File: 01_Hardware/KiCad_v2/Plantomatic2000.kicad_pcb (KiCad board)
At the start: 4 copper layers, 137.2 x 78 mm, 284 parts, among them J100 TYPE-C-31-M-12, J300 JST_B2B, J600 JST_B2B, J601 JST_B2B, J700 JST_B4B, J701 JST_B4B, J800 Conn_02x03_Odd_Even, J801 JST_B2B, J802 JST_B2B, J803 JST_B2B, J804 Conn_02x05_Odd_Even, J805 JST_B2B, J806 JST_B2B, J807 JST_B2B, J808 JST_B2B, Q100 UMH3N, Q200 SI7615DN-T1-GE3, Q201 SI7615DN-T1-GE3, Q202 DMP6050SSD, Q203 NVTA7002NT1G, Q300 BSS314PE, Q301 NVTA7002NT1G, Q400 SI7615DN-T1-GE3, Q401 SI7615DN-T1-GE3, Q402 NVTA7002NT1G, Q500 NVTA7002NT1G, Q600 STN3NF06L, Q601 STN3NF06L, Q700 BSS314PE, Q701 BSS314PE, Q702 NVTA7002NT1G, Q703 NVTA7002NT1G, SW800 SW_Push, SW801 SW_Push, U100 USBLC6-2P6, U101 CP2102N-A02-GQFN24, U200 CYPD3177-24LQ, U300 BQ25892, U400 BDJ2FC0WFP, U401 TLV61048, U402 NCP1117-12_SOT223, U403 XC6220B331MR, U404 XC6220B331MR, U500 DS3231M, U501 ESP32-WROOM-32E, U502 AT24CS01-SSHM

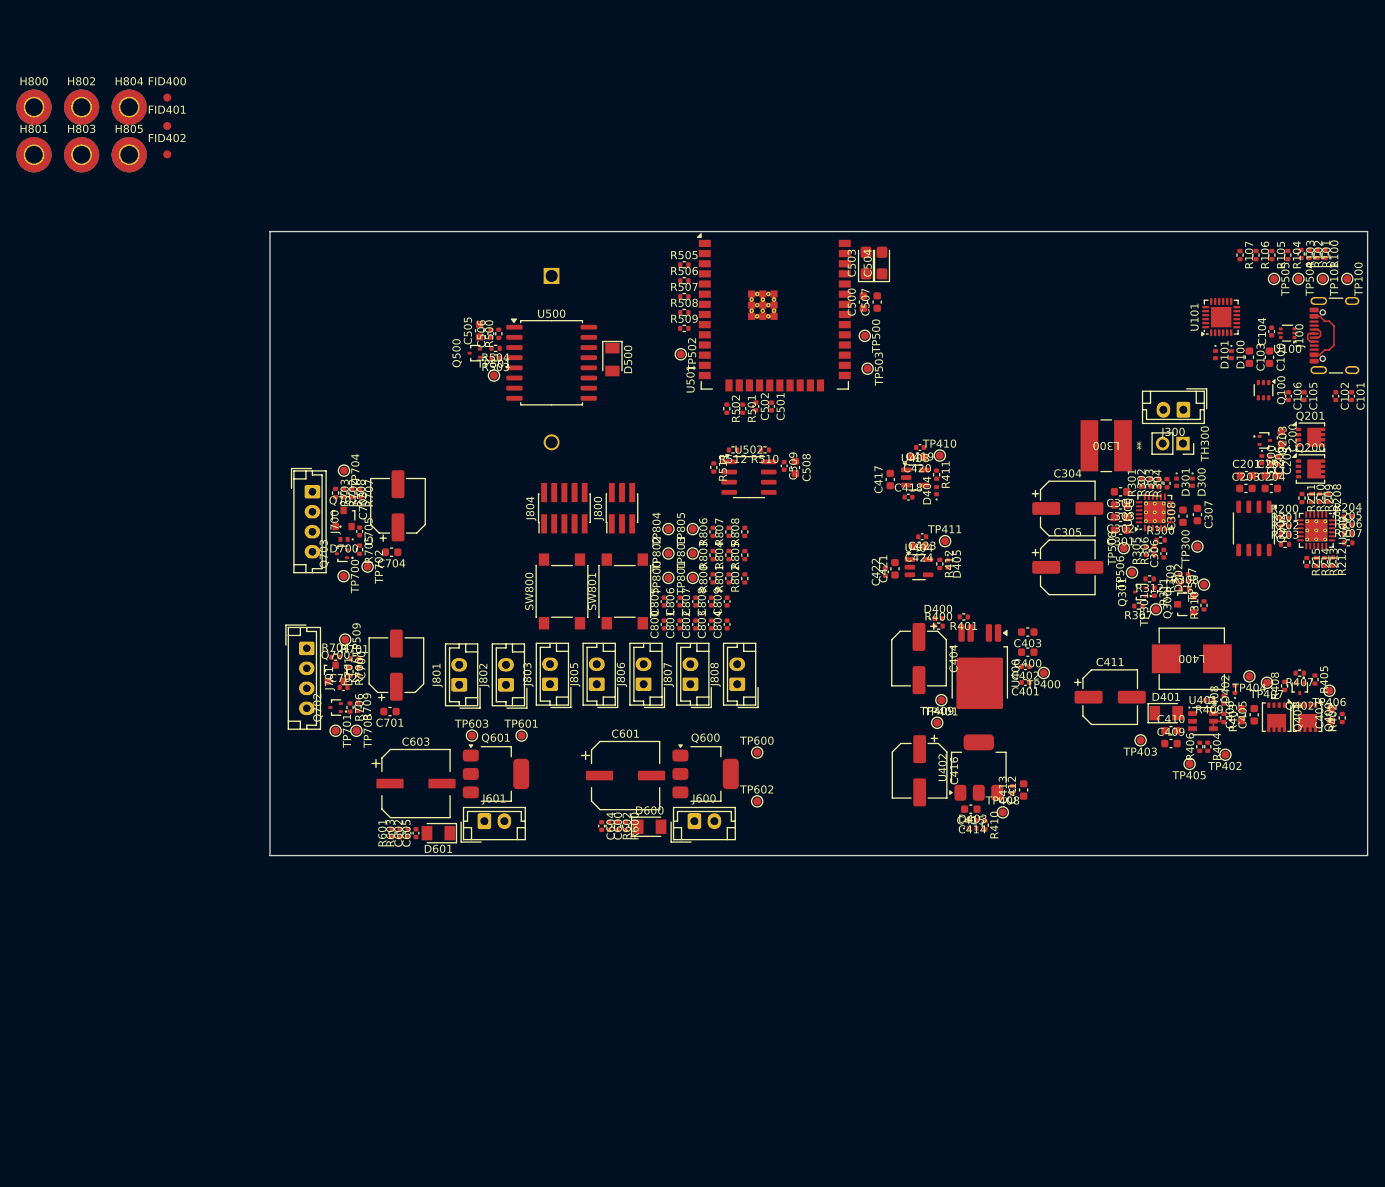
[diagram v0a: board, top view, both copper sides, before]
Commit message: USB-C and Serial PCB routing done
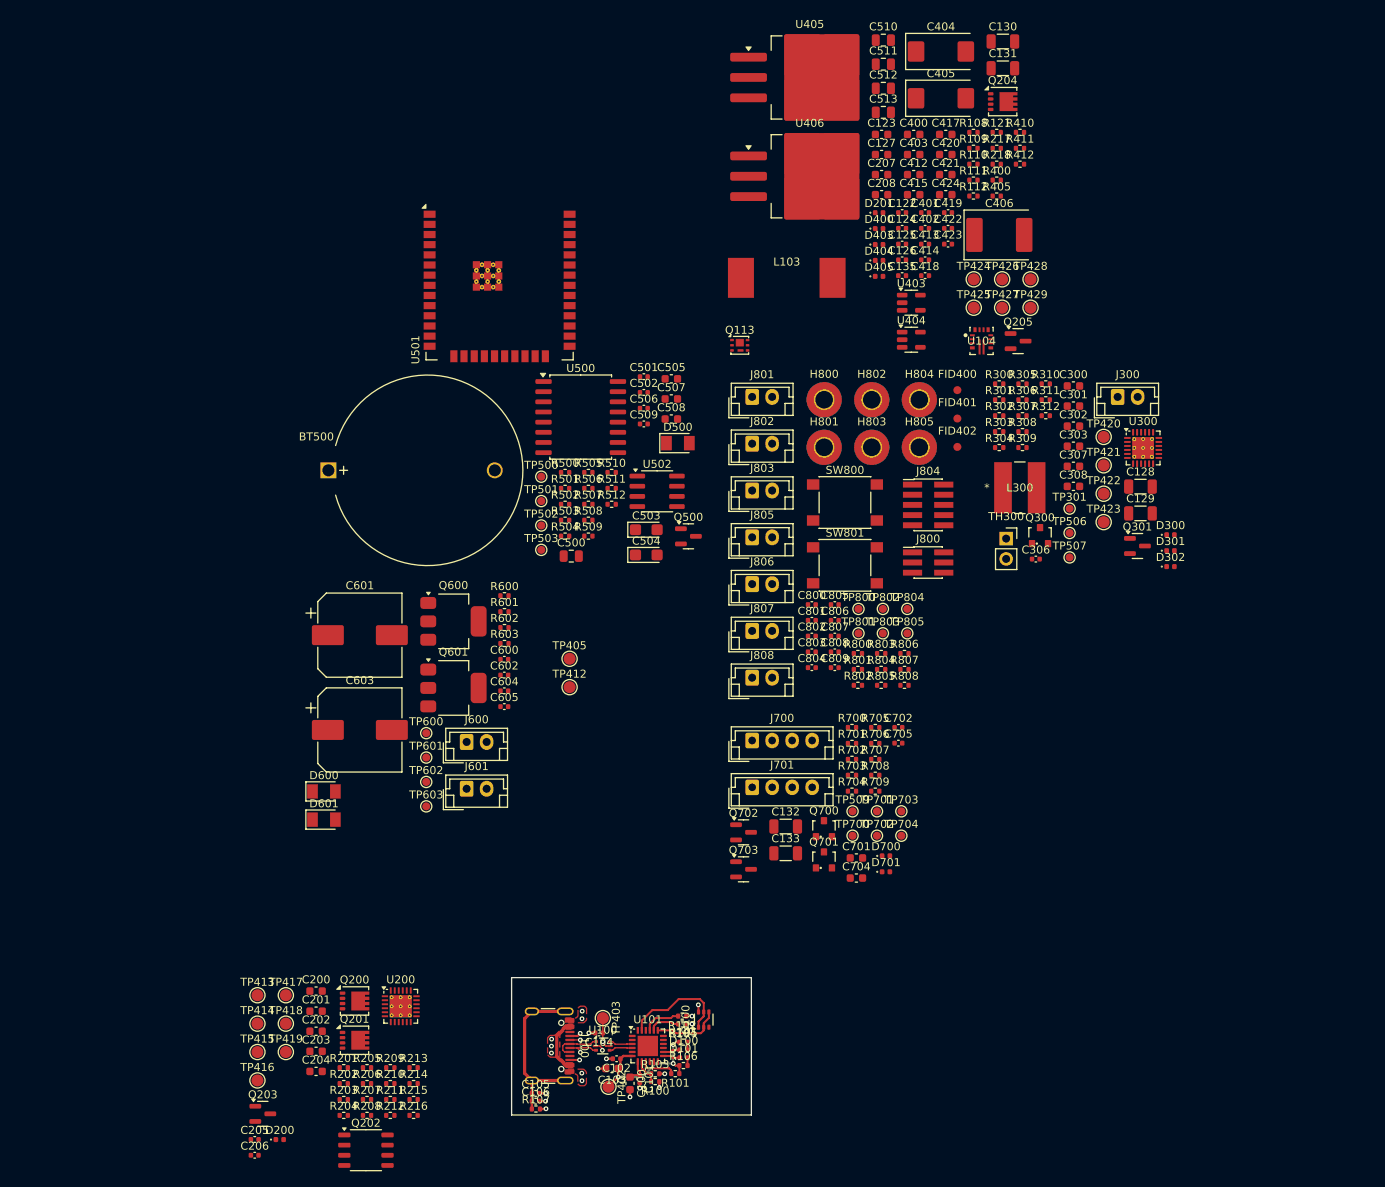
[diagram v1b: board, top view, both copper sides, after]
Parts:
- removed C304, C305, C411, C416, C700, C703: 47uF, Capacitor_SMD:CP_Elec_6.3x5.8
- removed C407, C409: 1uF, Capacitor_SMD:C_0603_1608Metric
- removed C408: 100nF, Capacitor_SMD:C_0402_1005Metric
- removed C410: 10uF, Capacitor_SMD:C_0603_1608Metric
- removed D401: SBR3U40S1F, Custom_Global_Footprints:SBR3U40S1F-7
- removed D402: NCD0402G1, Custom_Global_Footprints:SML-P13PTT_LED_0402_1005Metric
- removed L400: ETQ-P5M100YFM, Custom_Global_Footprints:ETQ-P5M100YFM
- removed Q400, Q401: SI7615DN-T1-GE3, Package_SON:Diodes_PowerDI3333-8
- removed Q402: NVTA7002NT1G, Custom_Global_Footprints:NVTA7002N
- removed R200, R401, R402, R403, R407: 10K, Resistor_SMD:R_0402_1005Metric
- removed R404: 1M, Resistor_SMD:R_0402_1005Metric
- removed R406: 64K9, Resistor_SMD:R_0402_1005Metric
- removed R408: 22K1, Resistor_SMD:R_0402_1005Metric
- removed R409: 1K, Resistor_SMD:R_0402_1005Metric
- removed TP100, TP101, TP404, TP406, TP407, TP410, TP411, TP504, TP505, TP508: ~, TestPoint:TestPoint_Pad_D1.0mm
- removed TP300: +VBAT, TestPoint:TestPoint_Pad_D1.0mm
- removed TP400, TP401, TP408, TP409: TestPoint_Small, TestPoint:TestPoint_Pad_D1.0mm
- removed U400: BDJ2FC0WFP, Package_TO_SOT_SMD:TO-252-4
- removed U401: TLV61048, Custom_Global_Footprints:TLV61048
- removed U402: NCP1117-12_SOT223, Package_TO_SOT_SMD:SOT-223
- added C122: 100nF, Capacitor_SMD:C_0402_1005Metric, F.Cu at (193.6, 46.5)
- added C123: 10uF, Capacitor_SMD:C_0603_1608Metric, F.Cu at (191.1, 36.8)
- added C124: 100nF, Capacitor_SMD:C_0402_1005Metric, F.Cu at (193.6, 48.5)
- added C125: 100pF, Capacitor_SMD:C_0402_1005Metric, F.Cu at (193.6, 50.5)
- added C126: 22nF, Capacitor_SMD:C_0402_1005Metric, F.Cu at (193.6, 52.4)
- added C127: 4.7uF, Capacitor_SMD:C_0603_1608Metric, F.Cu at (191.1, 39.3)
- added C128: 47uF, Capacitor_SMD:C_1206_3216Metric, F.Cu at (223.4, 80.8)
- added C129: 47uF, Capacitor_SMD:C_1206_3216Metric, F.Cu at (223.4, 84.1)
- added C130: 47uF, Capacitor_SMD:C_1206_3216Metric, F.Cu at (206.2, 25.1)
- added C131: 47uF, Capacitor_SMD:C_1206_3216Metric, F.Cu at (206.2, 28.5)
- added C132: 47uF, Capacitor_SMD:C_1206_3216Metric, F.Cu at (179.1, 123.3)
- added C133: 47uF, Capacitor_SMD:C_1206_3216Metric, F.Cu at (179.1, 126.6)
- added C135: 22nF, Capacitor_SMD:C_0402_1005Metric, F.Cu at (193.6, 54.4)
- added C207: 1uF, Capacitor_SMD:C_0603_1608Metric, F.Cu at (191.1, 41.8)
- added C208: 1uF, Capacitor_SMD:C_0603_1608Metric, F.Cu at (191.1, 44.3)
- added C510: 22uF, Capacitor_SMD:C_0805_2012Metric, F.Cu at (191.3, 25.0)
- added C511: 22uF, Capacitor_SMD:C_0805_2012Metric, F.Cu at (191.3, 28.0)
- added C512: 22uF, Capacitor_SMD:C_0805_2012Metric, F.Cu at (191.3, 31.0)
- added C513: 22uF, Capacitor_SMD:C_0805_2012Metric, F.Cu at (191.3, 34.0)
- added D201: NCD0402R1, LED_SMD:LED_0402_1005Metric, F.Cu at (190.7, 46.5)
- added L103: 4.7uH (SPM12565VT-4R7M-D), Custom_Global_Footprints:SPM12565VT-4R7M, F.Cu at (179.2, 54.7)
- added Q113: CSD17313Q2, Package_SON:Texas_DQK, F.Cu at (173.3, 63.1)
- added Q204: SI7615DN-T1-GE3, Package_SON:Diodes_PowerDI3333-8, F.Cu at (206.2, 32.7)
- added Q205: IRLML2402TRPBF, Package_TO_SOT_SMD:SOT-23, F.Cu at (208.1, 62.6)
- added R108: 158K, Resistor_SMD:R_0402_1005Metric, F.Cu at (202.5, 36.5)
- added R109: 14K3, Resistor_SMD:R_0402_1005Metric, F.Cu at (202.5, 38.5)
- added R110: 49K9, Resistor_SMD:R_0402_1005Metric, F.Cu at (202.5, 40.5)
- added R111: 20K, Resistor_SMD:R_0402_1005Metric, F.Cu at (202.5, 42.5)
- added R112: 22K1, Resistor_SMD:R_0402_1005Metric, F.Cu at (202.5, 44.5)
- added R121: 10K, Resistor_SMD:R_0402_1005Metric, F.Cu at (205.4, 36.5)
- added R216: 49K9, Resistor_SMD:R_0402_1005Metric, F.Cu at (132.6, 159.4)
- added R217: 49K9, Resistor_SMD:R_0402_1005Metric, F.Cu at (205.4, 38.5)
- added R218: 1K, Resistor_SMD:R_0402_1005Metric, F.Cu at (205.4, 40.5)
- added TP412: TestPoint_Small, TestPoint:TestPoint_Pad_D1.5mm, F.Cu at (152.1, 105.8)
- added TP413: TestPoint_Small, TestPoint:TestPoint_Pad_D1.5mm, F.Cu at (113.0, 144.4)
- added TP414: TestPoint_Small, TestPoint:TestPoint_Pad_D1.5mm, F.Cu at (113.0, 147.9)
- added TP415: TestPoint_Small, TestPoint:TestPoint_Pad_D1.5mm, F.Cu at (113.0, 151.5)
- added TP416: TestPoint_Small, TestPoint:TestPoint_Pad_D1.5mm, F.Cu at (113.0, 155.0)
- added TP417: TestPoint_Small, TestPoint:TestPoint_Pad_D1.5mm, F.Cu at (116.6, 144.4)
- added TP418: TestPoint_Small, TestPoint:TestPoint_Pad_D1.5mm, F.Cu at (116.6, 147.9)
- added TP419: TestPoint_Small, TestPoint:TestPoint_Pad_D1.5mm, F.Cu at (116.6, 151.5)
- added TP420: TestPoint_Small, TestPoint:TestPoint_Pad_D1.5mm, F.Cu at (218.8, 74.6)
- added TP421: TestPoint_Small, TestPoint:TestPoint_Pad_D1.5mm, F.Cu at (218.8, 78.1)
- added TP422: TestPoint_Small, TestPoint:TestPoint_Pad_D1.5mm, F.Cu at (218.8, 81.7)
- added TP423: TestPoint_Small, TestPoint:TestPoint_Pad_D1.5mm, F.Cu at (218.8, 85.2)
- added TP424: TestPoint_Small, TestPoint:TestPoint_Pad_D1.5mm, F.Cu at (202.6, 54.9)
- added TP425: TestPoint_Small, TestPoint:TestPoint_Pad_D1.5mm, F.Cu at (202.6, 58.4)
- added TP426: TestPoint_Small, TestPoint:TestPoint_Pad_D1.5mm, F.Cu at (206.1, 54.9)
- added TP427: TestPoint_Small, TestPoint:TestPoint_Pad_D1.5mm, F.Cu at (206.1, 58.4)
- added TP428: TestPoint_Small, TestPoint:TestPoint_Pad_D1.5mm, F.Cu at (209.7, 54.9)
- added TP429: TestPoint_Small, TestPoint:TestPoint_Pad_D1.5mm, F.Cu at (209.7, 58.4)
- added U104: TPS61287RZPR, Custom_Global_Footprints:RZP0014A-MFG, F.Cu at (203.5, 62.6)
- added U405: LM1085IS-12/NOPB, Package_TO_SOT_SMD:TO-263-3_TabPin2, F.Cu at (182.1, 29.6)
- added U406: LM1085IS-12/NOPB, Package_TO_SOT_SMD:TO-263-3_TabPin2, F.Cu at (182.1, 42.0)
- BT500: moved to F.Cu
- C404: value 47uF -> 330uF; footprint Capacitor_SMD:CP_Elec_6.3x5.8 -> Capacitor_Tantalum_SMD:CP_EIA-7343-31_Kemet-D
- C405: value 1uF -> 330uF; footprint Capacitor_SMD:C_0603_1608Metric -> Capacitor_Tantalum_SMD:CP_EIA-7343-31_Kemet-D
- C406: value 1uF -> 470uF; footprint Capacitor_SMD:C_0603_1608Metric -> Capacitor_Tantalum_SMD:CP_EIA-7360-38_Kemet-E
- C500: footprint Capacitor_SMD:C_0603_1608Metric -> Capacitor_SMD:C_0805_2012Metric
- C601, C603: footprint Custom_Global_Footprints:EEEFK1V470P -> Capacitor_SMD:CP_Elec_10x10
- D100, D101, D200, D300, D301, D302, D400, D403, D404, D405, D700, D701: footprint Custom_Global_Footprints:SML-P13PTT_LED_0402_1005Metric -> LED_SMD:LED_0402_1005Metric
- Q202: value DMP6050SSD -> DMP6050SSD-13
- Q203, Q301, Q500, Q702, Q703: value NVTA7002NT1G -> IRLML2402TRPBF; footprint Custom_Global_Footprints:NVTA7002N -> Package_TO_SOT_SMD:SOT-23
- Q300, Q700, Q701: value BSS314PE -> BSS314PEH6327
- TP402, TP403, TP405: footprint TestPoint:TestPoint_Pad_D1.0mm -> TestPoint:TestPoint_Pad_D1.5mm
- U101: value CP2102N-A02-GQFN24 -> CP2102N-A02-GQFN24R
- U403, U404: value XC6220B331MR -> XC6220B331MR-G
- U501: value ESP32-WROOM-32E -> ESP32-WROOM-32E-N4
- moved C206 153.8 mm to (112.7, 164.4), turned to 0 degrees
- moved C205 153.5 mm to (112.7, 162.4), turned to 0 degrees
- moved Q203 150.9 mm to (113.7, 159.2), turned to 0 degrees
- moved D200 149.3 mm to (115.8, 162.4), turned to 0 degrees
- moved R204 146.1 mm to (123.8, 159.4)
- moved R208 142.8 mm to (126.7, 159.4), turned to 0 degrees
- moved Q201 141.3 mm to (125.2, 150.0)
- moved R207 141.0 mm to (126.7, 157.4)
- moved R206 140.6 mm to (126.7, 155.4)
- moved R205 140.1 mm to (126.7, 153.4)
- moved C204 139.9 mm to (120.4, 153.9)
- moved C200 139.1 mm to (120.4, 143.8), turned to 0 degrees
- moved R107 138.3 mm to (147.8, 158.6), turned to 0 degrees
- moved C202 138.1 mm to (120.4, 148.9)
- moved Q200 136.8 mm to (125.2, 145.1)
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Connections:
- C404 pad 1: +12V_PUMP -> Net-(Q204-D)
- C405 pad 1: Net-(Q401-D) -> +12V
- C405 pad 2: Net-(Q400-G) -> GND
- C406 pad 1: Net-(Q401-D) -> +12V
- TP402 pad 1: Net-(Q401-D) -> +VDD
- TP403 pad 1: /DC_DC_REGULATORS/BOOST_IND -> +VBUS
- TP405 pad 1: Net-(U401-FB) -> /USB_C_TO_SERIAL/DTR_SERIAL
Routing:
- net Net-(J100-SHIELD): track 0.00 -> 21.3 mm
- net +VDD: track 0.00 -> 18.5 mm, vias 0 -> 3
- net /USB_C_TO_SERIAL/DTR_SERIAL: track 0.00 -> 13.6 mm
- net /USB_C_TO_SERIAL/RTS_SERIAL: track 0.00 -> 8.61 mm
- net GND: track 0.00 -> 8.37 mm, vias 0 -> 14
- net +VBUS: track 8.70 -> 14.9 mm, vias 0 -> 5
- net /USB_C_TO_SERIAL/SER_TX: track 0.00 -> 4.76 mm
- net /USB_C_TO_SERIAL/USB_CONN_D-: track 2.34 -> 7.01 mm, vias 0 -> 2
- net /USB_C_TO_SERIAL/RST: track 0.00 -> 4.42 mm
- net /USB_C_TO_SERIAL/SER_RX: track 0.00 -> 3.89 mm
- net /USB_C_TO_SERIAL/USB_CONN_D+: track 2.31 -> 5.92 mm
- net /USB_C_TO_SERIAL/VBUS_VDIV: track 0.00 -> 3.25 mm
- net /USB_C_TO_SERIAL/USB_D+: track 0.00 -> 2.96 mm
- net /USB_C_TO_SERIAL/USB_D-: track 0.00 -> 2.96 mm
- net Net-(Q401-D): track 2.30 -> 0.00 mm
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- added copper zone on F.Cu, net +VBUS
- added copper zone on F.Cu, net GND
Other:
- board size 137.2 x 78 mm -> 30 x 17.2 mm

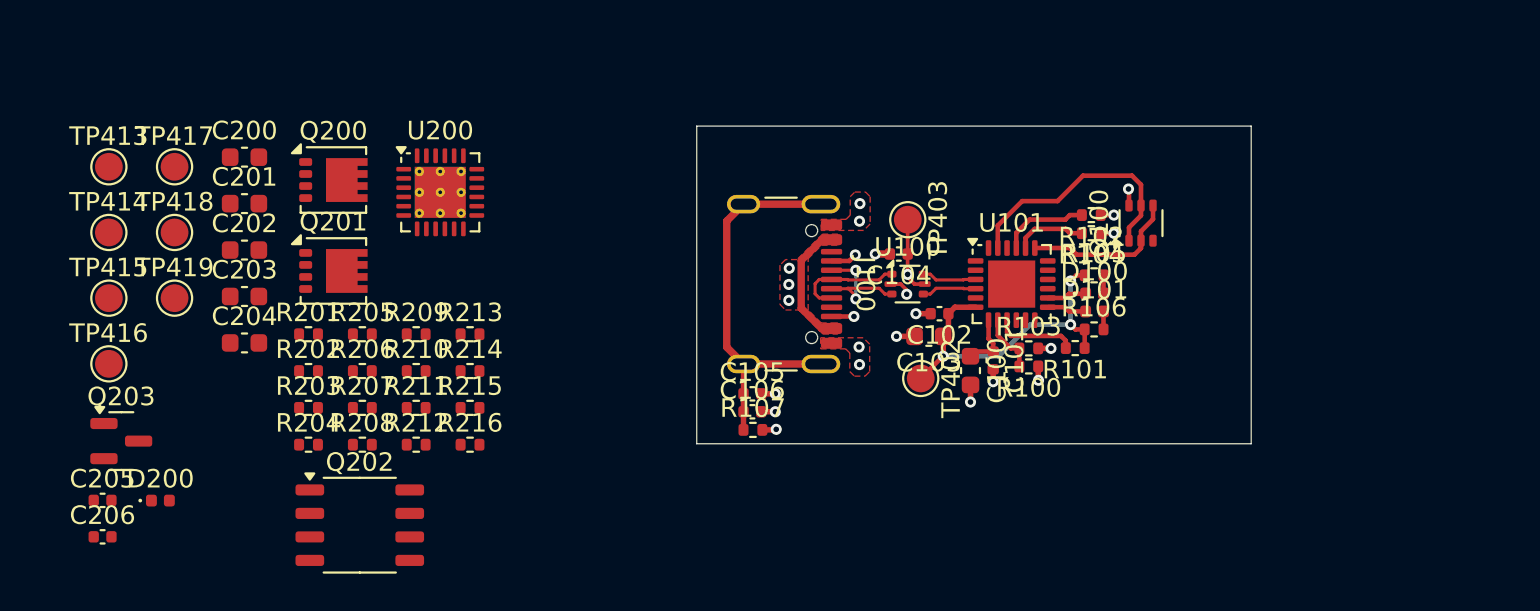
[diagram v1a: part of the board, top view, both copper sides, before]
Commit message: PCB desing in progresssss
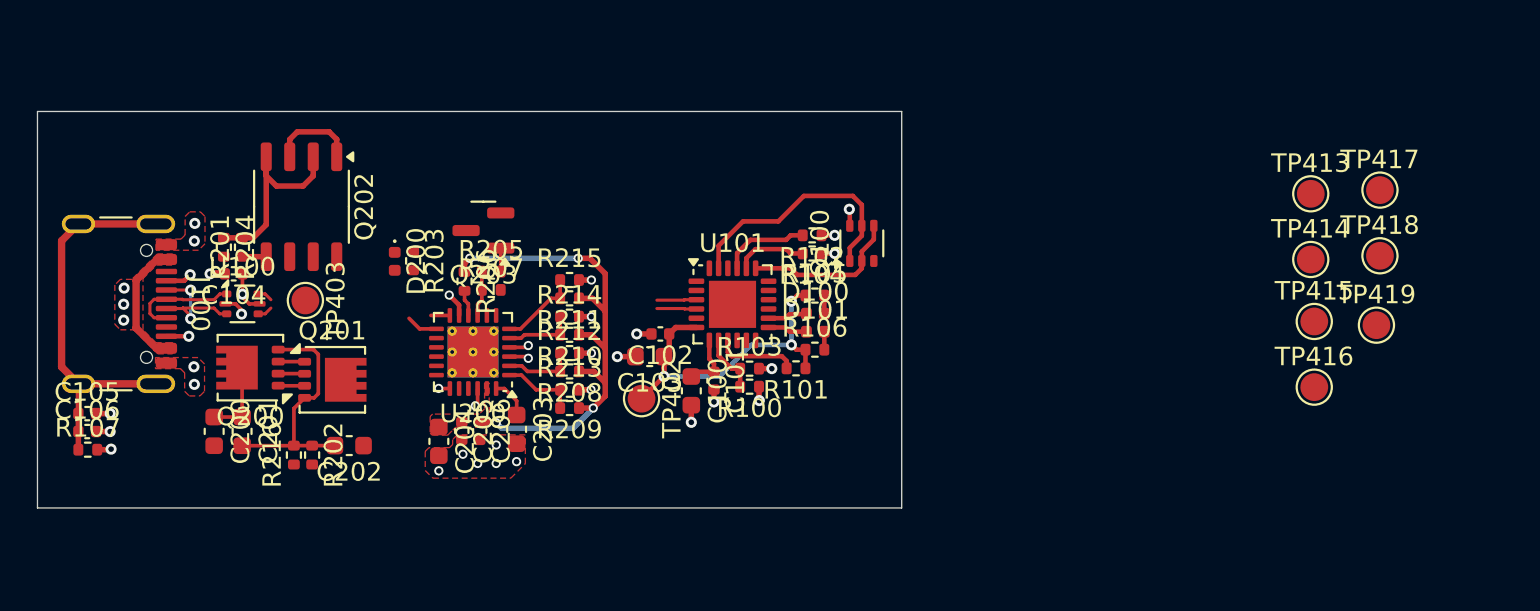
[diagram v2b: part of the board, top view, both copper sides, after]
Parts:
- moved TP415 65.2 mm to (178.2, 152.7)
- moved TP416 65.2 mm to (178.2, 156.3)
- moved TP417 65.2 mm to (181.7, 145.6)
- moved TP418 65.2 mm to (181.7, 149.2)
- moved TP413 65.0 mm to (178.0, 145.8)
- moved TP414 65.0 mm to (178.0, 149.4)
- moved TP419 65.0 mm to (181.5, 152.9)
- moved C105 36.0 mm to (111.9, 157.7)
- moved C106 36.0 mm to (111.9, 158.7)
- moved J100 36.0 mm to (112.5, 151.8)
- moved R107 36.0 mm to (111.9, 159.7)
- moved C104 36.0 mm to (119.8, 150.1)
- moved U100 36.0 mm to (120.2, 151.8)
- moved TP403 32.9 mm to (123.7, 151.6)
- moved Q203 22.6 mm to (133.3, 147.8), turned to 180 degrees
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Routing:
- net +VDDD: track 0.00 -> 28.6 mm, vias 0 -> 4
- net /USB_C_POWER_DELIVERY/VBUS_FET_EN: track 0.00 -> 13.1 mm
- net /BATTERY_MANAGEMENT_IC/VBUS_FET_SAFE_EN: track 0.00 -> 11.3 mm
- net Net-(Q202A-S1): track 0.00 -> 4.76 mm
- net /USB_C_POWER_DELIVERY/ISNK_FINE: track 0.00 -> 4.41 mm
- net Net-(Q200-S-Pad1): track 0.00 -> 4.29 mm
- net GND: track 8.37 -> 12.6 mm, vias 14 -> 26
- net /USB_C_POWER_DELIVERY/VBUS_MIN: track 0.00 -> 4.05 mm
- net /USB_C_POWER_DELIVERY/VBUS_MAX: track 0.00 -> 3.85 mm
- net /USB_C_POWER_DELIVERY/ISNK_COARSE: track 0.00 -> 3.79 mm
- net +VBUS: track 14.9 -> 18.5 mm
- net /USB_C_POWER_DELIVERY/FAULT: track 0.00 -> 2.46 mm
- net /USB_C_POWER_DELIVERY/VCCD: track 0.00 -> 2.15 mm
- net ESP_SCL: track 0.00 -> 1.72 mm
- net Net-(U200-FLIP): track 0.00 -> 1.42 mm
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- added copper zone on F.Cu, net +VDDD
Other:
- board size 30 x 17.2 mm -> 46.7 x 21.4 mm
